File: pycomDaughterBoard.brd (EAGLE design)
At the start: 40.3 x 50.8 mm, 18 parts, among them J1 BilgeSwitch, J2 Button, J3 LED, J4 VCC

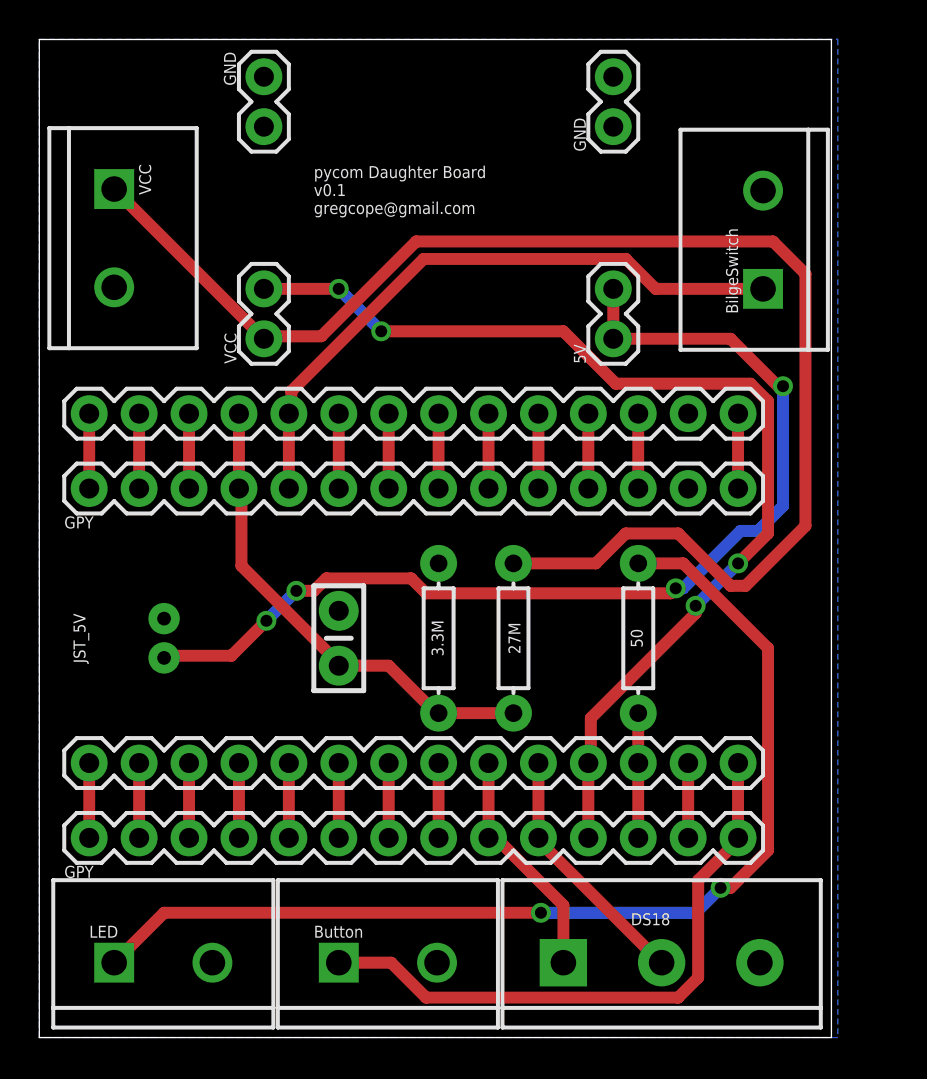
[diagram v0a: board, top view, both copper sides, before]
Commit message: new v0.3 board
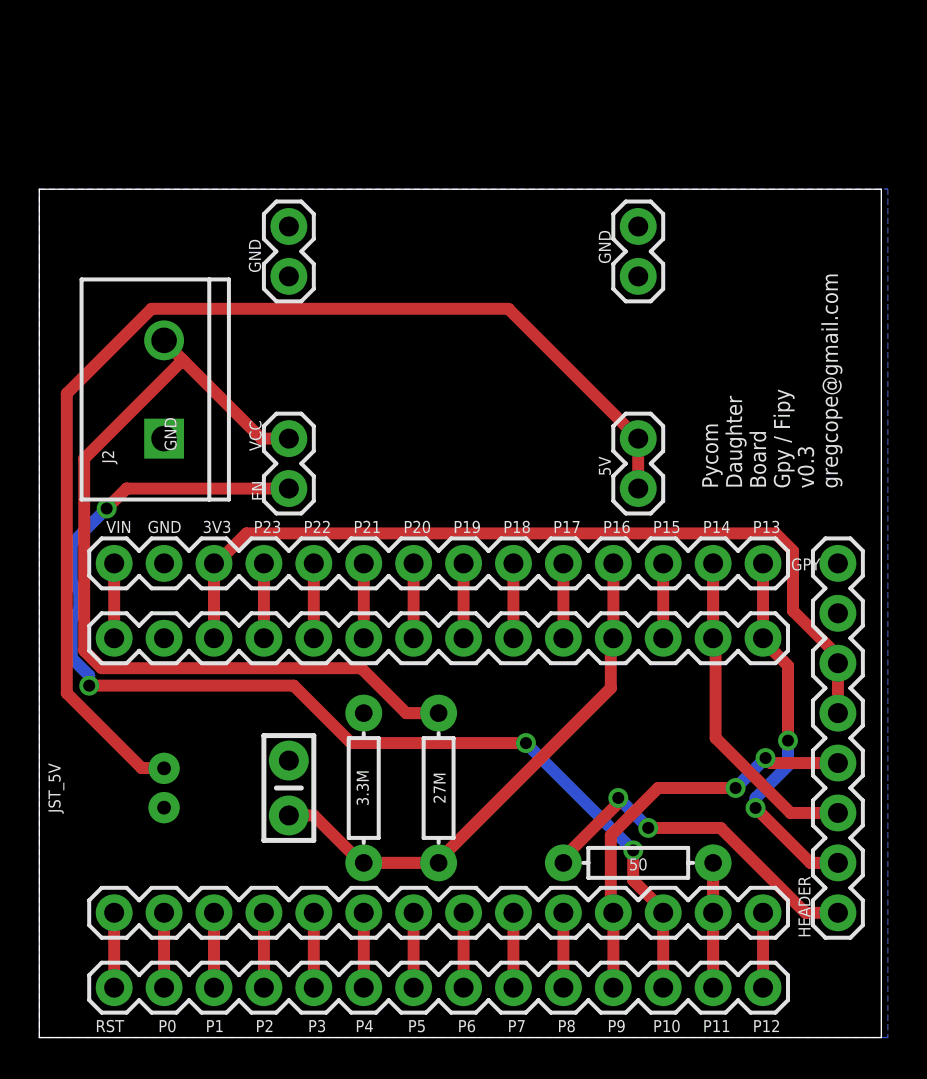
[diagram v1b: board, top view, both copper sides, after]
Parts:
- removed DS18: DS18, SparkFun-Connectors:SCREWTERMINAL-5MM-3
- removed GPY, GPY1, GPY_II1: GPY, SparkFun-Connectors:1X14
- removed J1: BilgeSwitch, SparkFun-Retired:SCREWTERMINAL-5MM-2
- removed J3: LED, SparkFun-Retired:SCREWTERMINAL-5MM-2
- removed J4: VCC, SparkFun-Retired:SCREWTERMINAL-5MM-2
- added 12, PY: RST, SparkFun-Connectors:1X14
- added HEADER: J1, SparkFun-Connectors:1X08
- added VIN: GPY, SparkFun-Connectors:1X14
- J2: value Button -> VCC
- JST_5V: value JST_5V -> 5v
- moved GPY_II 36.1 mm to (36.8, 20.3), turned to 180 degrees
- moved J2 28.1 mm to (6.35, 30.5), turned to 90 degrees
- moved R7 11.4 mm to (30.5, 8.89), turned to 0 degrees
- moved R2 8.52 mm to (20.3, 12.7)
- moved R3 8.52 mm to (16.5, 12.7)
- moved C1 8.03 mm to (12.7, 12.7)
- moved GND_II 7.73 mm to (12.7, 41.3)
- moved 5V 7.73 mm to (30.5, 27.9)
- moved VCC 7.73 mm to (12.7, 27.9)
- moved GND 7.73 mm to (30.5, 38.7)
- moved JST_5V 7.62 mm to (6.35, 12.7)
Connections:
- removed net N$19: GPY_II.6, GPY_II1.6
- removed net N$21: GPY_II.2, GPY_II1.2
- removed net N$22: GPY_II.1, GPY_II1.1
- removed net P12: GPY.12, GPY1.12, R7.P$2
- removed net P19: GPY_II.5, GPY_II1.5, J1.1
- new net 3V3: GPY_II.12, HEADER.5, HEADER.6, VIN.12
- new net N$12: GPY_II.9, VIN.9
- new net P13: GPY_II.1, HEADER.2, VIN.1
- new net P16: C1.1, GPY_II.4, R2.P$1, R3.P$2, VIN.4
- new net P17: GPY_II.5, VIN.5
- net 5V: now also JST_5V.2; no longer JST_5V.1
- net GND: now also HEADER.7, HEADER.8, J2.1, JST_5V.1, VIN.13; no longer DS18.3, GPY_II1.13, J1.2, J2.2, J3.2, J4.2, JST_5V.2
- net N$1: now also 12.1, PY.1; no longer GPY.1, GPY1.1
- net N$10: now also 12.9, PY.9; no longer GPY.13, GPY1.13
- net N$11: now also VIN.14; no longer GPY_II1.14
- net N$13: now also 12.10, PY.10; no longer GPY_II.12, GPY_II1.12
- net N$14: now also VIN.11; no longer GPY_II1.11
- net N$15: now also VIN.10; no longer GPY_II1.10
- net N$16: now also 12.14, PY.14; no longer GPY_II.9, GPY_II1.9
- net N$17: now also VIN.8; no longer GPY_II1.8
- net N$18: now also VIN.7; no longer GPY_II1.7
- net N$2: now also HEADER.1; no longer J3.1
- net N$20: now also VIN.3; no longer GPY_II1.3
- net N$3: now also 12.2, PY.2; no longer GPY.2, GPY1.2
- net N$4: now also 12.3, PY.3; no longer GPY.3, GPY1.3
- net N$5: now also 12.4, PY.4; no longer GPY.4, GPY1.4
- net N$6: now also 12.5, PY.5; no longer GPY.5, GPY1.5
- net N$7: now also 12.6, PY.6; no longer GPY.6, GPY1.6
- net N$8: now also 12.7, PY.7; no longer GPY.7, GPY1.7
- net N$9: now also 12.8, PY.8; no longer GPY.8, GPY1.8
- net P10: now also 12.12, PY.12, VCC.1; no longer DS18.2, GPY.10, GPY1.10
- net P11: now also 12.13, PY.13, R7.P$2; no longer GPY.11, GPY1.11, VCC.2
- net P14: now also GPY_II.2, HEADER.3, VIN.2; no longer GPY.14, GPY1.14, J2.1
- net P18: now also GPY_II.6, VIN.6; no longer C1.1, GPY_II.4, GPY_II1.4, R2.P$1, R3.P$2
- net P9: now also 12.11, HEADER.4, PY.11; no longer DS18.1, GPY.9, GPY1.9
- net VCC: now also J2.2, VCC.2; no longer J4.1, VCC.1
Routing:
- net P11: track 54.0 -> 6.35 mm, vias 4 -> 0
- net P10: track 12.8 -> 58.9 mm, vias 0 -> 4
- net 3V3: track 0.00 -> 43.4 mm
- net N$2: track 54.3 -> 18.1 mm
- net P19: track 32.4 -> 0.00 mm
- net P16: track 0.00 -> 27.5 mm
- net VCC: track 71.7 -> 44.7 mm
- net P18: track 24.8 -> 3.81 mm
- net P13: track 0.00 -> 19.0 mm, vias 0 -> 2
- net P14: track 31.2 -> 16.7 mm
- net P9: track 12.0 -> 21.1 mm, vias 0 -> 2
- net P12: track 6.35 -> 0.00 mm
- net 5V: track 53.7 -> 57.9 mm, vias 4 -> 0
- net P17: track 0.00 -> 3.81 mm
- net N$22: track 3.81 -> 0.00 mm
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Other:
- board size 40.3 x 50.8 mm -> 42.9 x 43.2 mm
- board text added: "3V3"
- board text added: "EN"
- board text added: "GND"
- board text added: "P0"
- board text added: "P1"
- board text added: "P10"
- board text added: "P11"
- board text added: "P12"
- board text added: "P13"
- board text added: "P14"
- board text added: "P15"
- board text added: "P16"
- board text added: "P17"
- board text added: "P18"
- board text added: "P19"
- board text added: "P2"
- board text added: "P20"
- board text added: "P21"
- board text added: "P22"
- board text added: "P23"
- board text added: "P3"
- board text added: "P4"
- board text added: "P5"
- board text added: "P6"
- board text added: "P7"
- board text added: "P8"
- board text added: "P9"
- board text added: "Pycom Daughter Board Gpy / Fipy v0.3 gregcope@gmail.com"
- board text added: "RST"
- board text added: "VIN"
- board text removed: "pycom Daughter Board v0.1 gregcope@gmail.com"
